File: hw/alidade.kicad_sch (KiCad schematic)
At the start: 0 parts

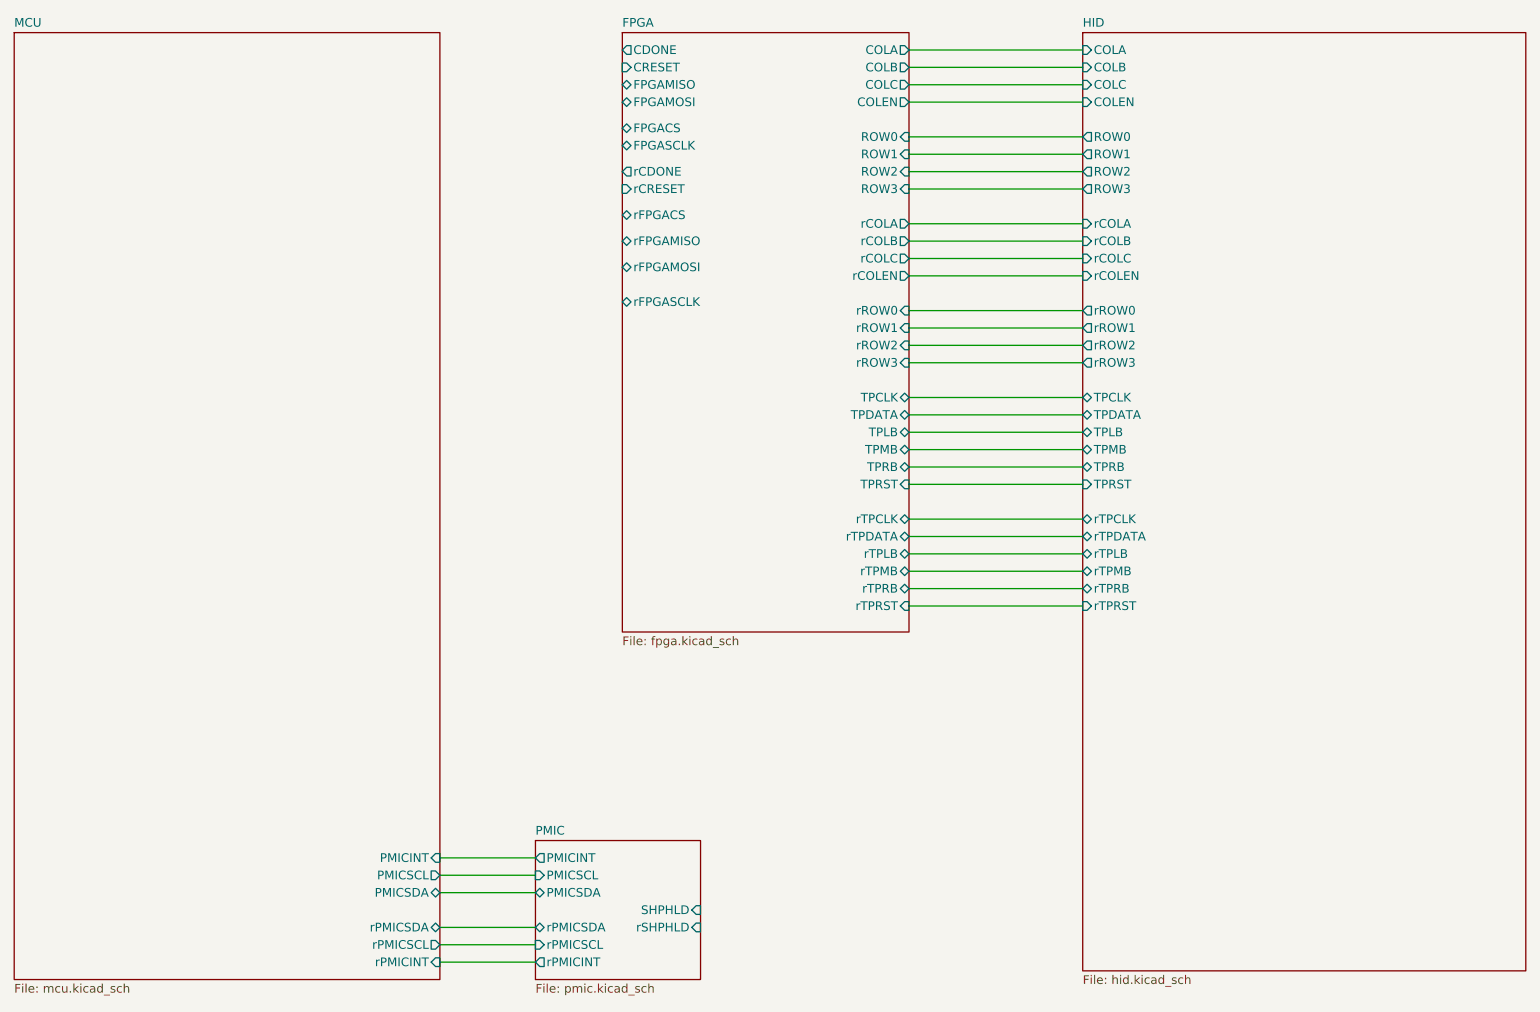
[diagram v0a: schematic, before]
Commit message: Sheet pins
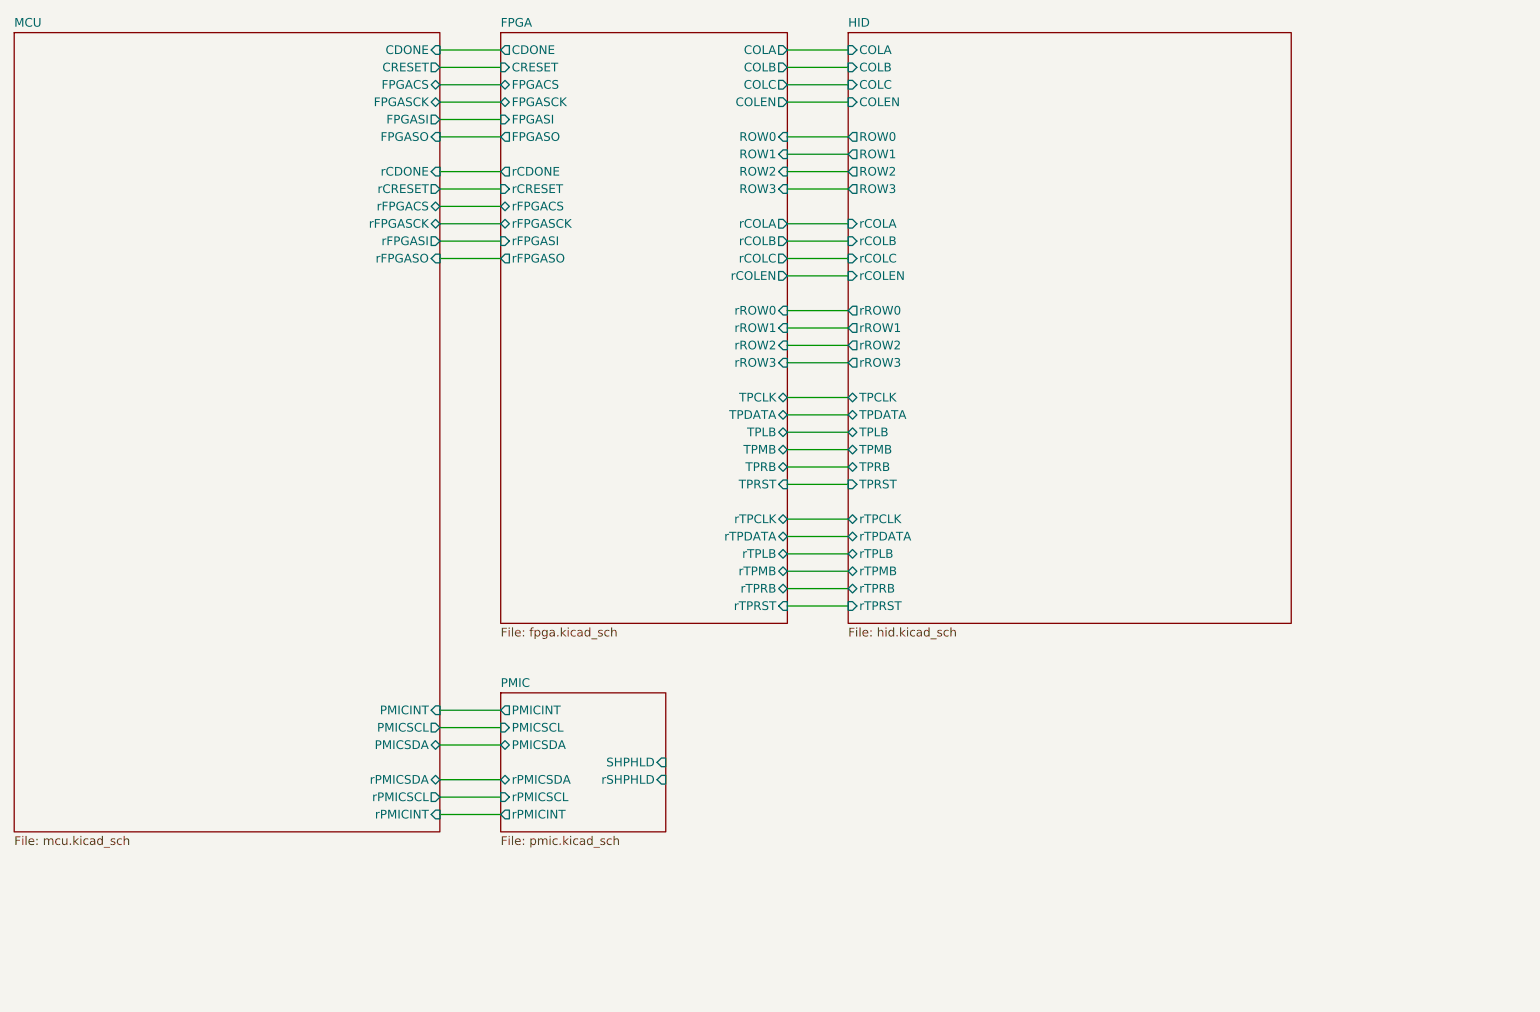
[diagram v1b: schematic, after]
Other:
- sheet FPGA ports: added FPGASCK, FPGASI, FPGASO, rFPGASCK, rFPGASI, rFPGASO; removed FPGAMISO, FPGAMOSI, FPGASCLK, rFPGAMISO, rFPGAMOSI, rFPGASCLK
- sheet MCU ports: added CDONE, CRESET, FPGACS, FPGASCK, FPGASI, FPGASO, rCDONE, rCRESET, rFPGACS, rFPGASCK, rFPGASI, rFPGASO; removed none
